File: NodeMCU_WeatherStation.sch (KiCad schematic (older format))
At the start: 24 parts, among them J12 Screw_Terminal_01x02, J14 Screw_Terminal_01x02, J15 Conn_01x10, J4 Conn_01x04, J5 Conn_01x04, U1 BME280, U7 R-785.0-0.5

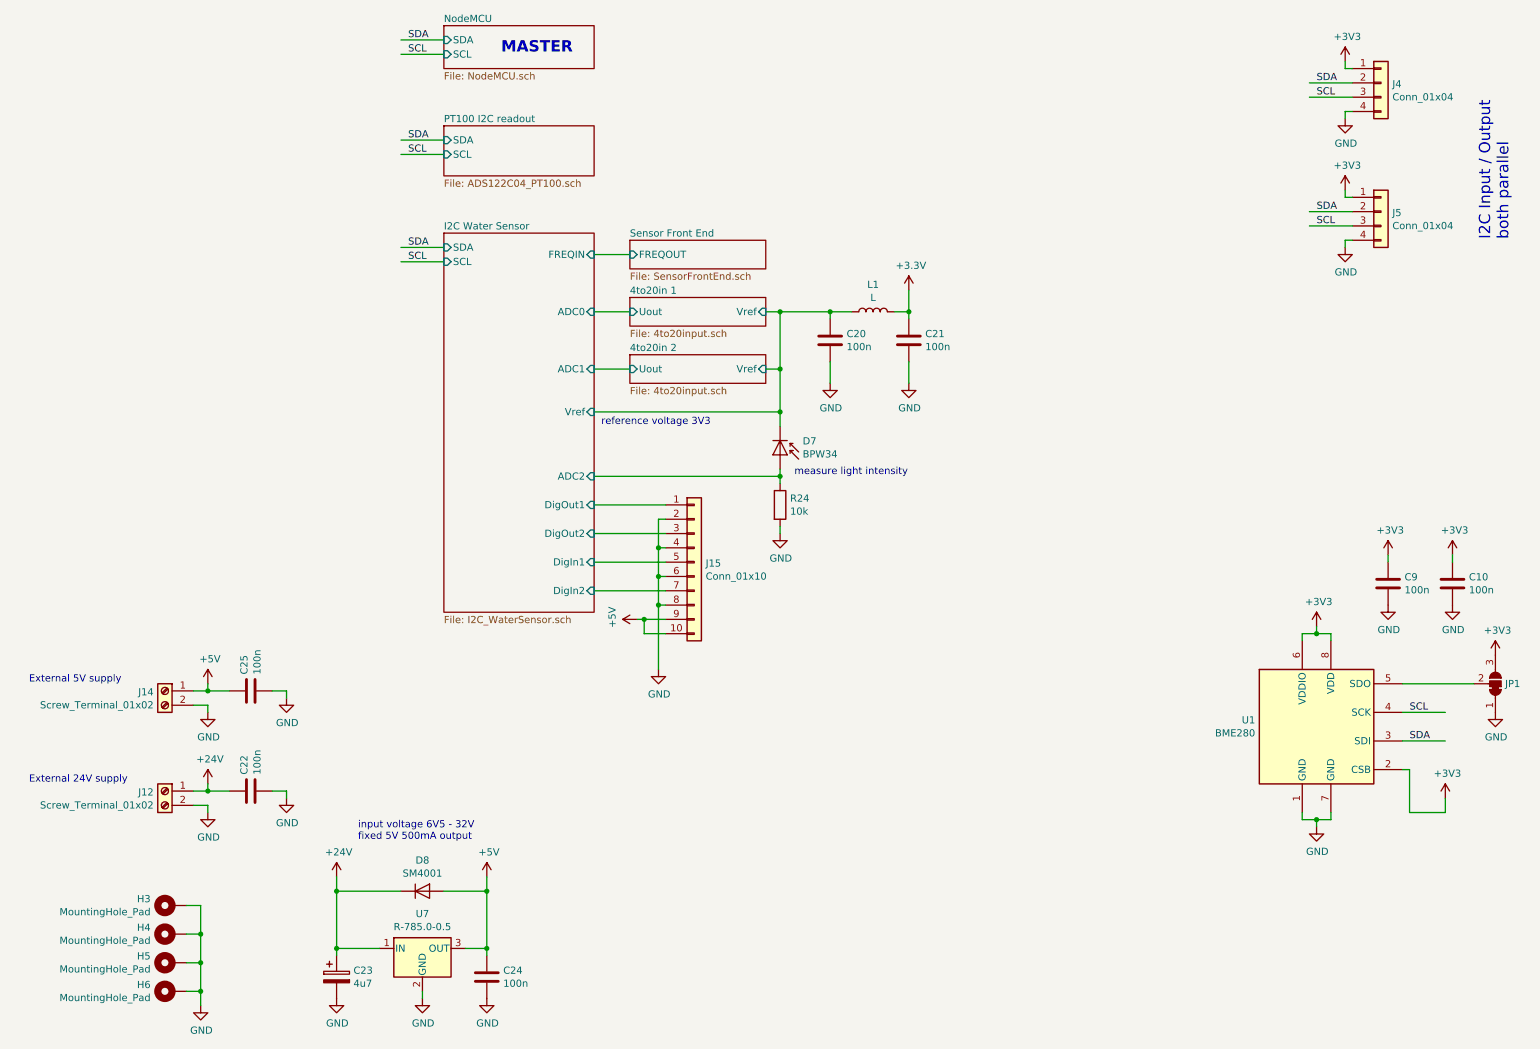
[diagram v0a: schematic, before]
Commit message: include latest changes
latest changes to design
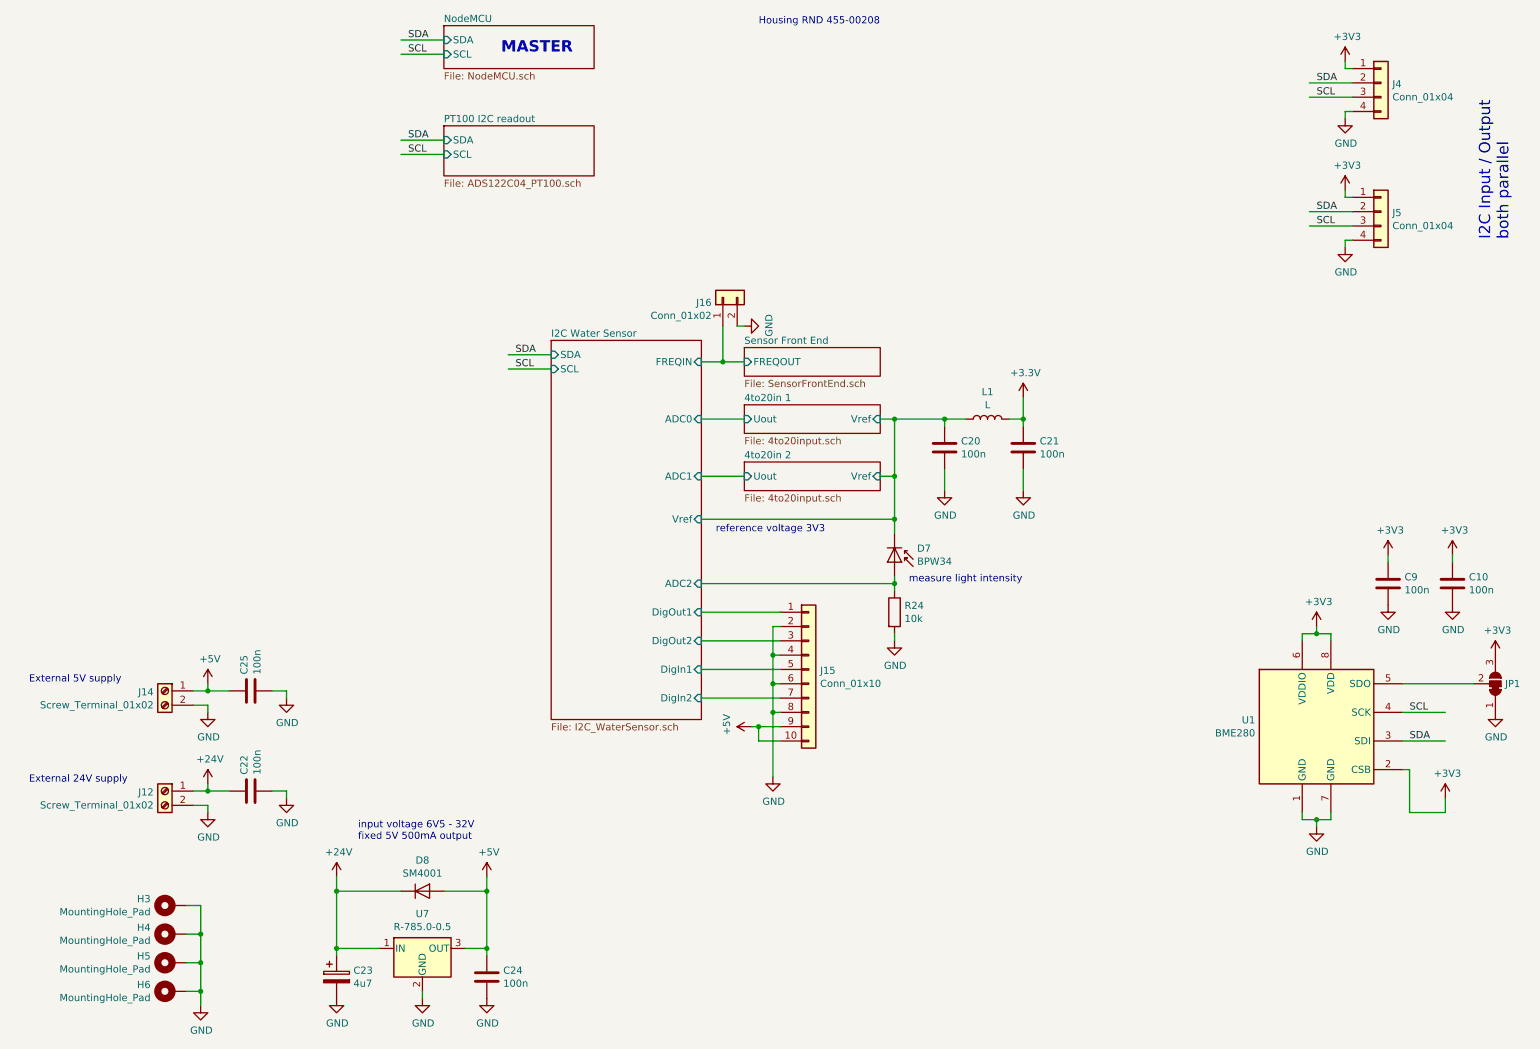
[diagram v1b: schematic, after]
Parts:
- added J16: Conn_01x02, Connector_PinHeader_2.54mm:PinHeader_1x02_P2.54mm_Vertical, symbol Connector_Generic:Conn_01x02
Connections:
- wire segments 107 -> 110
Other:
- note added: "Housing RND 455-00208"
- moved on the sheet: C20, C21, D7, J15, L1, R24
